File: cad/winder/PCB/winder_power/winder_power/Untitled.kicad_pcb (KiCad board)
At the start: 2 copper layers, 40 x 51 mm, 22 parts, among them M3 MountingHole_3.2mm_M3, Q1 IRF4905

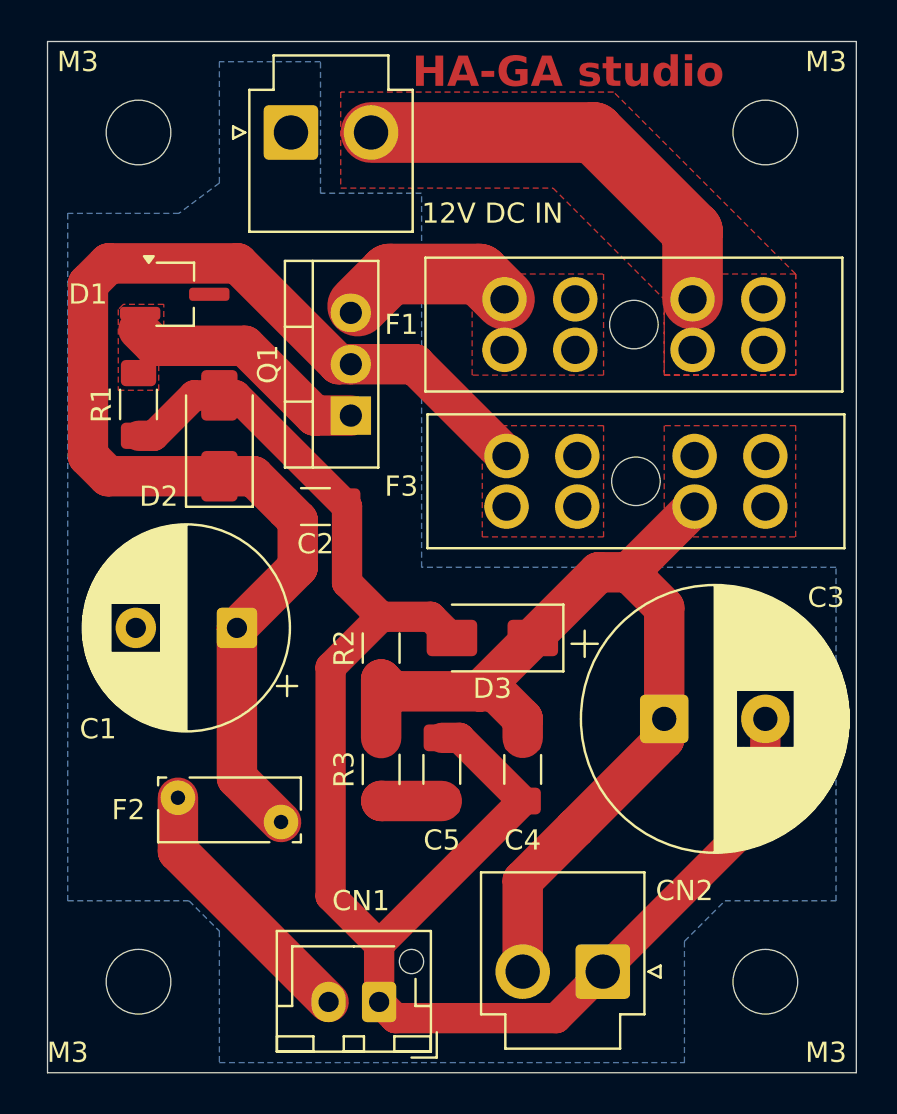
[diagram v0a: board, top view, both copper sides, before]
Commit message: パーツリストMDを作成
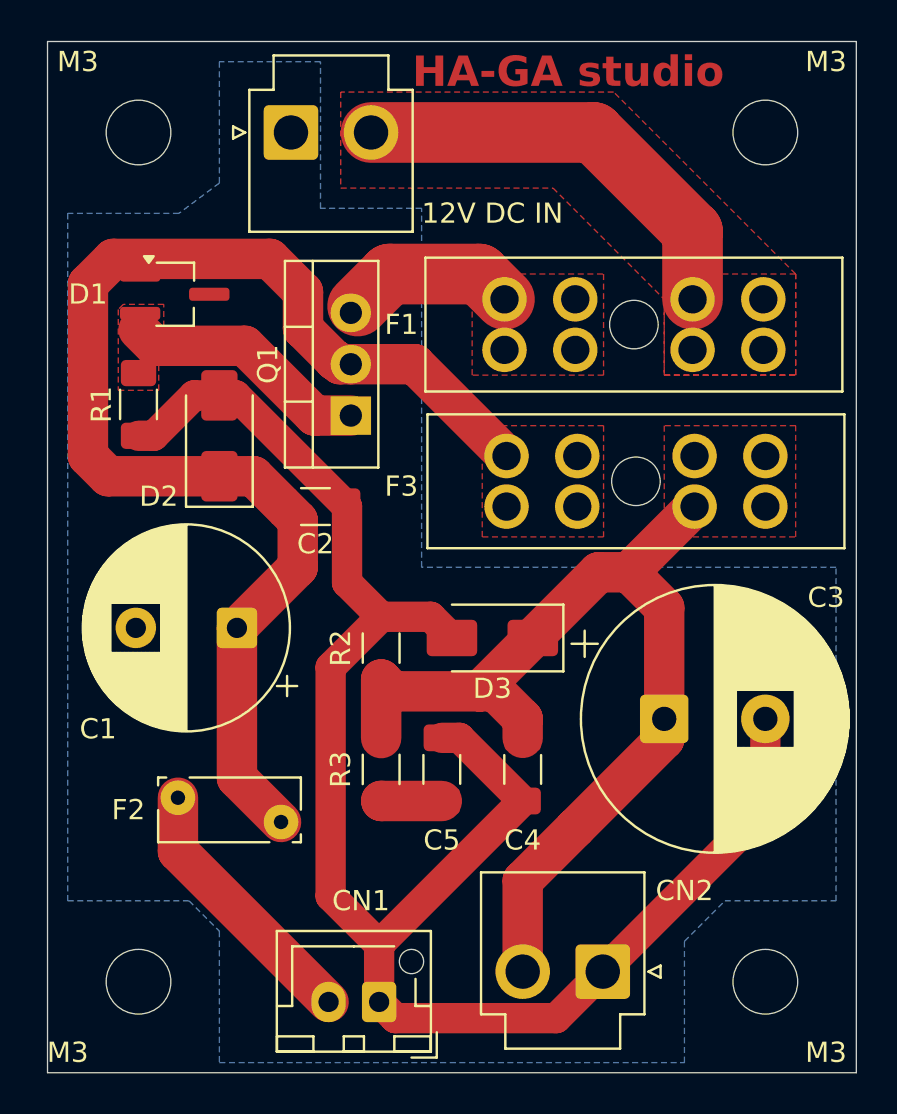
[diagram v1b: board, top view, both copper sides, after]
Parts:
- turned C5 to -90 degrees
- turned R2 to -90 degrees
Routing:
- net GND: track 91.1 -> 88.1 mm
- net Net-(C5-Pad2): track 0.00 -> 3.01 mm
- net /fuse post 12V: track 62.3 -> 63.6 mm
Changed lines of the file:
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@@
 			(outputformat 1)
 			(mirror no)
-			(drillshape 1)
+			(drillshape 0)
 			(scaleselection 1)
-			(outputdirectory "")
+			(outputdirectory "../../../../../../guiter_winder_gerber/power_pcb/")
 		)
 	)
@@
 		(tags "resistor handsolder")
 		(property "Reference" "R3"
-			(at 0 -1.83 90)
+			(at 0 -2 90)
 			(layer "F.SilkS")
 			(effects
@@
 	(footprint "Capacitor_SMD:C_1206_3216Metric_Pad1.33x1.80mm_HandSolder"
 		(layer "F.Cu")
-		(at 140 93 90)
+		(at 140 93 -90)
 		(descr "Capacitor SMD 1206 (3216 Metric), square (rectangular) end terminal, IPC-7351 nominal with elongated pad for handsoldering. (Body size source: IPC-SM-782 page 76, https://www.pcb-3d.com/wordpress/wp-content/uploads/ipc-sm-782a_amendment_1_and_2.pdf), generated with kicad-footprint-generator")
 		(tags "capacitor handsolder")
 		(property "Reference" "C5"
-			(at -3.5 0 180)
+			(at 3.5 0 180)
 			(layer "F.SilkS")
 			(effects
@@
 		(attr smd)
 		(fp_line
-			(start -0.711252 -0.91)
-			(end 0.711252 -0.91)
+			(start -0.711252 0.91)
+			(end 0.711252 0.91)
 			(stroke
 				(width 0.12)
@@
 		)
 		(fp_line
-			(start -0.711252 0.91)
-			(end 0.711252 0.91)
+			(start -0.711252 -0.91)
+			(end 0.711252 -0.91)
 			(stroke
 				(width 0.12)
@@
 		)
 		(fp_line
-			(start 2.48 -1.15)
-			(end 2.48 1.15)
+			(start -2.48 1.15)
+			(end -2.48 -1.15)
 			(stroke
 				(width 0.05)
@@
 		)
 		(fp_line
-			(start -2.48 -1.15)
-			(end 2.48 -1.15)
+			(start 2.48 1.15)
+			(end -2.48 1.15)
 			(stroke
 				(width 0.05)
@@
 		)
 		(fp_line
-			(start 2.48 1.15)
-			(end -2.48 1.15)
+			(start -2.48 -1.15)
+			(end 2.48 -1.15)
 			(stroke
 				(width 0.05)
@@
 		)
 		(fp_line
-			(start -2.48 1.15)
-			(end -2.48 -1.15)
+			(start 2.48 -1.15)
+			(end 2.48 1.15)
 			(stroke
 				(width 0.05)
@@
 		)
 		(fp_line
-			(start 1.6 -0.8)
-			(end 1.6 0.8)
+			(start -1.6 0.8)
+			(end -1.6 -0.8)
 			(stroke
 				(width 0.1)
@@
 		)
 		(fp_line
-			(start -1.6 -0.8)
-			(end 1.6 -0.8)
+			(start 1.6 0.8)
+			(end -1.6 0.8)
 			(stroke
 				(width 0.1)
@@
 		)
 		(fp_line
-			(start 1.6 0.8)
-			(end -1.6 0.8)
+			(start -1.6 -0.8)
+			(end 1.6 -0.8)
 			(stroke
 				(width 0.1)
@@
 		)
 		(fp_line
-			(start -1.6 0.8)
-			(end -1.6 -0.8)
+			(start 1.6 -0.8)
+			(end 1.6 0.8)
 			(stroke
 				(width 0.1)
@@
 		)
 		(pad "1" smd roundrect
-			(at -1.5625 0 90)
+			(at -1.5625 0 270)
 			(size 1.325 1.8)
 			(layers "F.Cu" "F.Mask" "F.Paste")
@@
 		)
 		(pad "2" smd roundrect
-			(at 1.5625 0 90)
+			(at 1.5625 0 270)
 			(size 1.325 1.8)
 			(layers "F.Cu" "F.Mask" "F.Paste")
@@
 	(footprint "Resistor_SMD:R_1206_3216Metric_Pad1.30x1.75mm_HandSolder"
 		(layer "F.Cu")
-		(at 137 87 90)
+		(at 137 87 -90)
 		(descr "Resistor SMD 1206 (3216 Metric), square (rectangular) end terminal, IPC-7351 nominal with elongated pad for handsoldering. (Body size source: IPC-SM-782 page 72, https://www.pcb-3d.com/wordpress/wp-content/uploads/ipc-sm-782a_amendment_1_and_2.pdf), generated with kicad-footprint-generator")
 		(tags "resistor handsolder")
 		(property "Reference" "R2"
-			(at 0 -1.83 90)
+			(at 0 2 90)
 			(layer "F.SilkS")
 			(effects
@@
 		(attr smd)
 		(fp_line
-			(start -0.727064 -0.91)
-			(end 0.727064 -0.91)
+			(start -0.727064 0.91)
+			(end 0.727064 0.91)
 			(stroke
 				(width 0.12)
@@
 		)
 		(fp_line
-			(start -0.727064 0.91)
-			(end 0.727064 0.91)
+			(start -0.727064 -0.91)
+			(end 0.727064 -0.91)
 			(stroke
 				(width 0.12)
@@
 		)
 		(fp_line
-			(start 2.45 -1.13)
-			(end 2.45 1.13)
+			(start -2.45 1.13)
+			(end -2.45 -1.13)
 			(stroke
 				(width 0.05)
@@
 		)
 		(fp_line
-			(start -2.45 -1.13)
-			(end 2.45 -1.13)
+			(start 2.45 1.13)
+			(end -2.45 1.13)
 			(stroke
 				(width 0.05)
@@
 		)
 		(fp_line
-			(start 2.45 1.13)
-			(end -2.45 1.13)
+			(start -2.45 -1.13)
+			(end 2.45 -1.13)
 			(stroke
 				(width 0.05)
@@
 		)
 		(fp_line
-			(start -2.45 1.13)
-			(end -2.45 -1.13)
+			(start 2.45 -1.13)
+			(end 2.45 1.13)
 			(stroke
 				(width 0.05)
@@
 		)
 		(fp_line
-			(start 1.6 -0.8)
-			(end 1.6 0.8)
+			(start -1.6 0.8)
+			(end -1.6 -0.8)
 			(stroke
 				(width 0.1)
@@
 		)
 		(fp_line
-			(start -1.6 -0.8)
-			(end 1.6 -0.8)
+			(start 1.6 0.8)
+			(end -1.6 0.8)
 			(stroke
 				(width 0.1)
@@
 		)
 		(fp_line
-			(start 1.6 0.8)
-			(end -1.6 0.8)
+			(start -1.6 -0.8)
+			(end 1.6 -0.8)
 			(stroke
 				(width 0.1)
@@
 		)
 		(fp_line
-			(start -1.6 0.8)
-			(end -1.6 -0.8)
+			(start 1.6 -0.8)
+			(end 1.6 0.8)
 			(stroke
 				(width 0.1)
@@
 		)
 		(pad "1" smd roundrect
-			(at -1.55 0 90)
+			(at -1.55 0 270)
 			(size 1.3 1.75)
 			(layers "F.Cu" "F.Mask" "F.Paste")
@@
 		)
 		(pad "2" smd roundrect
-			(at 1.55 0 90)
+			(at 1.55 0 270)
 			(size 1.3 1.75)
 			(layers "F.Cu" "F.Mask" "F.Paste")
@@
 	)
 	(segment
-		(start 140 91.4375)
-		(end 140.875 91.4375)
-		(width 1.5)
-		(layer "F.Cu")
-		(net 1)
-	)
-	(segment
 		(start 140.875 91.4375)
 		(end 144 94.5625)
@@
 	)
 	(segment
-		(start 137.0125 94.5625)
-		(end 137 94.55)
-		(width 2)
-		(layer "F.Cu")
-		(net 1)
-	)
-	(segment
-		(start 140 94.5625)
-		(end 137.0125 94.5625)
-		(width 2)
-		(layer "F.Cu")
-		(net 1)
-	)
-	(segment
 		(start 129.8125 74.5)
 		(end 135.3125 80)
@@
 	)
 	(segment
+		(start 140 91.4375)
+		(end 140.875 91.4375)
+		(width 1.5)
+		(layer "F.Cu")
+		(net 1)
+	)
+	(segment
 		(start 137 85.45)
 		(end 139.45 85.45)
@@
 	)
 	(segment
-		(start 129.906784 67.974)
-		(end 134.892784 72.96)
+		(start 137.0125 94.5625)
+		(end 137 94.55)
+		(width 2)
+		(layer "F.Cu")
+		(net 4)
+	)
+	(segment
+		(start 140 94.5625)
+		(end 137.0125 94.5625)
+		(width 2)
+		(layer "F.Cu")
+		(net 4)
+	)
+	(segment
+		(start 134.784713 72.784713)
+		(end 134.96 72.96)
 		(width 2)
 		(layer "F.Cu")
@@
 	)
 	(segment
-		(start 122.5 69)
-		(end 123.526 67.974)
+		(start 133.135287 71.202503)
+		(end 134.717497 72.784713)
 		(width 2)
 		(layer "F.Cu")
@@
 	)
 	(segment
-		(start 123.526 67.974)
-		(end 129.906784 67.974)
+		(start 123.75 67.75)
+		(end 131.5 67.75)
 		(width 2)
 		(layer "F.Cu")
@@
 	)
 	(segment
-		(start 129.867677 93.417677)
-		(end 132.05 95.6)
+		(start 122.5 77.5)
+		(end 122.5 69)
 		(width 2)
 		(layer "F.Cu")
@@
 	)
 	(segment
-		(start 129 78.5)
-		(end 123.5 78.5)
+		(start 129.867677 93.417677)
+		(end 132.05 95.6)
 		(width 2)
 		(layer "F.Cu")
@@
 	)
 	(segment
+		(start 123.5 78.5)
+		(end 122.5 77.5)
+		(width 2)
+		(layer "F.Cu")
+		(net 5)
+	)
+	(segment
 		(start 138.66 72.96)
 		(end 143.2 77.5)
@@
 	)
 	(segment
-		(start 130.6875 78.5)
-		(end 132.875 80.6875)
+		(start 133.135287 69.385287)
+		(end 133.135287 71.202503)
 		(width 2)
 		(layer "F.Cu")
@@
 	)
 	(segment
-		(start 122.5 77.5)
-		(end 122.5 69)
+		(start 134.96 72.96)
+		(end 135.5 72.96)
 		(width 2)
 		(layer "F.Cu")
@@
 	)
 	(segment
-		(start 134.892784 72.96)
-		(end 135.5 72.96)
+		(start 130.6875 78.5)
+		(end 132.875 80.6875)
+		(width 2)
+		(layer "F.Cu")
+		(net 5)
+	)
+	(segment
+		(start 131.5 67.75)
+		(end 133.135287 69.385287)
 		(width 2)
 		(layer "F.Cu")
@@
 	)
 	(segment
-		(start 123.5 78.5)
-		(end 122.5 77.5)
+		(start 122.5 69)
+		(end 123.75 67.75)
+		(width 2)
+		(layer "F.Cu")
+		(net 5)
+	)
+	(segment
+		(start 134.717497 72.784713)
+		(end 134.784713 72.784713)
 		(width 2)
 		(layer "F.Cu")
@@
 	)
 	(segment
+		(start 129 78.5)
+		(end 123.5 78.5)
+		(width 2)
+		(layer "F.Cu")
+		(net 5)
+	)
+	(segment
 		(start 126.95 97.05)
 		(end 134.4 104.5)
@@
 				(xy 129 58) (xy 129 64) (xy 127 65.5) (xy 121.5 65.5) (xy 121.5 99.5) (xy 127.5 99.5) (xy 129 101)
 				(xy 129 107.5) (xy 152 107.5) (xy 152 101.5) (xy 154 99.5) (xy 159.5 99.5) (xy 159.5 83) (xy 139 83)
-				(xy 139 64.5) (xy 134 64.5) (xy 134 58)
+				(xy 139 65.25) (xy 134 65.25) (xy 134 58)
 			)
 		)

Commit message: Fix winder asset naming and BOM units
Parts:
- C4: value 0.1mF -> 0.1uF
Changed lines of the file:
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@@
 			(drillshape 0)
 			(scaleselection 1)
-			(outputdirectory "../../../../../../guiter_winder_gerber/power_pcb/")
+			(outputdirectory "../../../../../../guitar_winder_gerber/power_pcb/")
 		)
 	)
@@
 			)
 		)
-		(property "Value" "0.1mF"
+		(property "Value" "0.1uF"
 			(at 0 1.85 90)
 			(layer "F.Fab")
